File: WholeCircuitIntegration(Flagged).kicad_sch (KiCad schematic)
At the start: 18 parts, among them J1 Conn_02x20_Odd_Even, J2 Conn_01x03_Socket, J3 Conn_01x03_Socket, J4 Conn_01x03_Socket, J5 Conn_01x03_Socket, J6 TBP03R2-350-03BE, J7 TBP03R2-350-03BE, J8 TBP03R2-350-03BE, J9 TBP03R2-350-03BE, U1 ADS1115IDGS, U2 BNO055, U3 74LV14

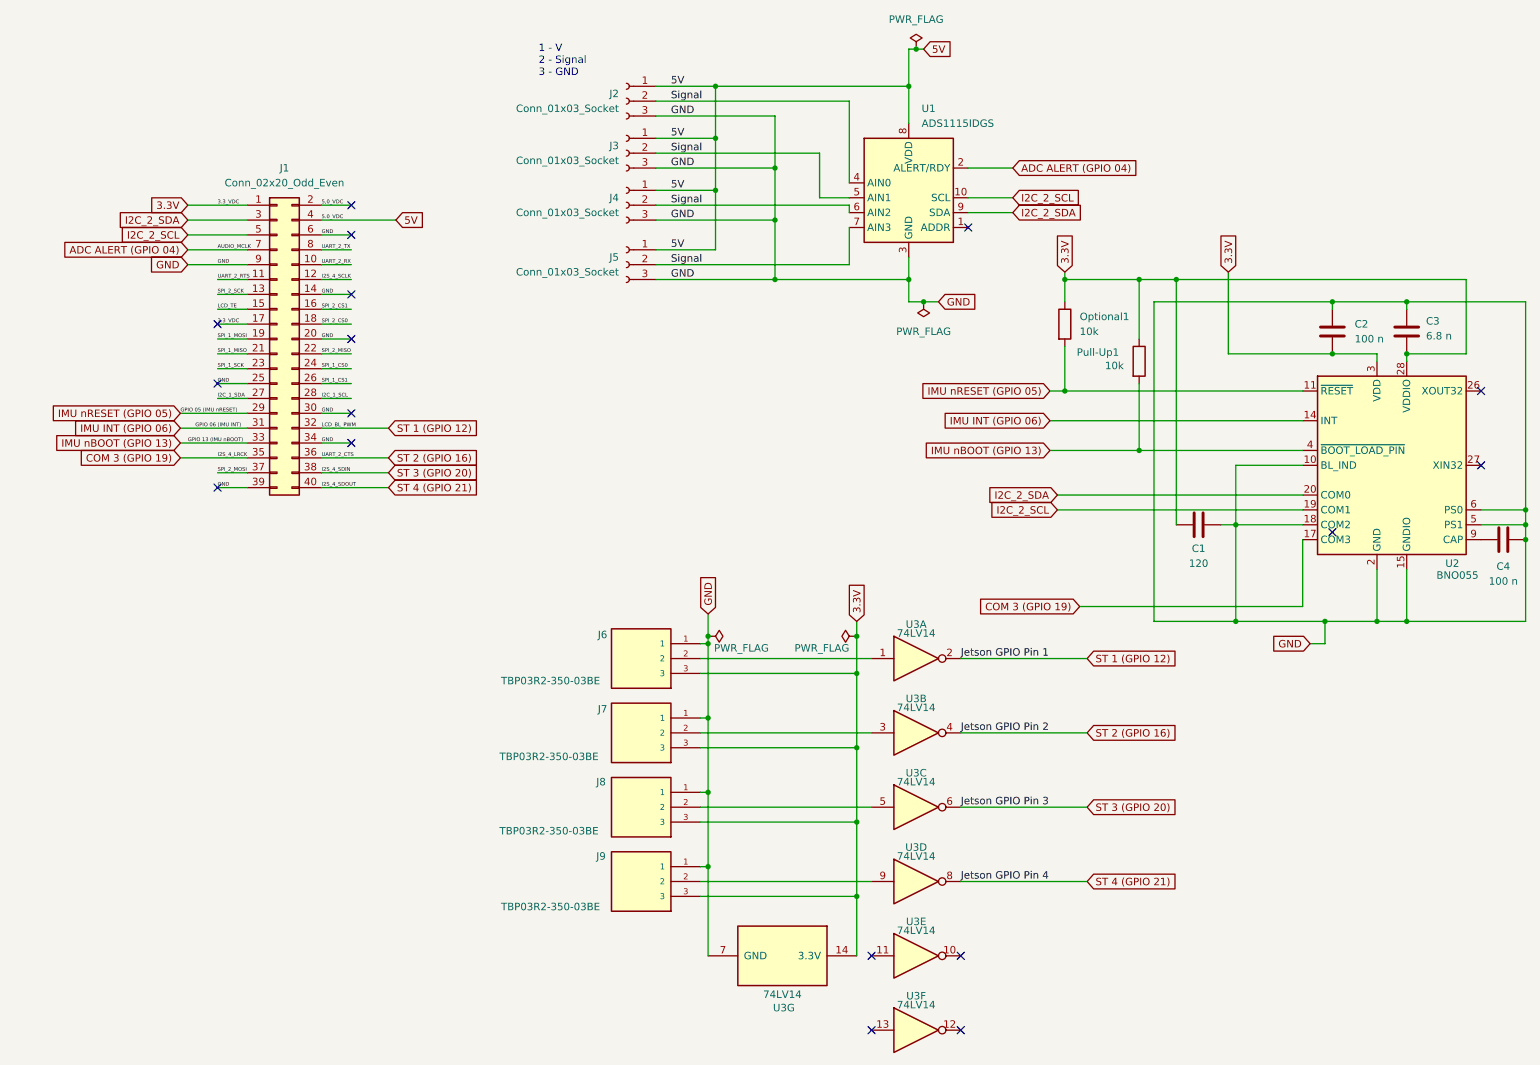
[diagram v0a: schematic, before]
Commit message: Whole Circuit Integration
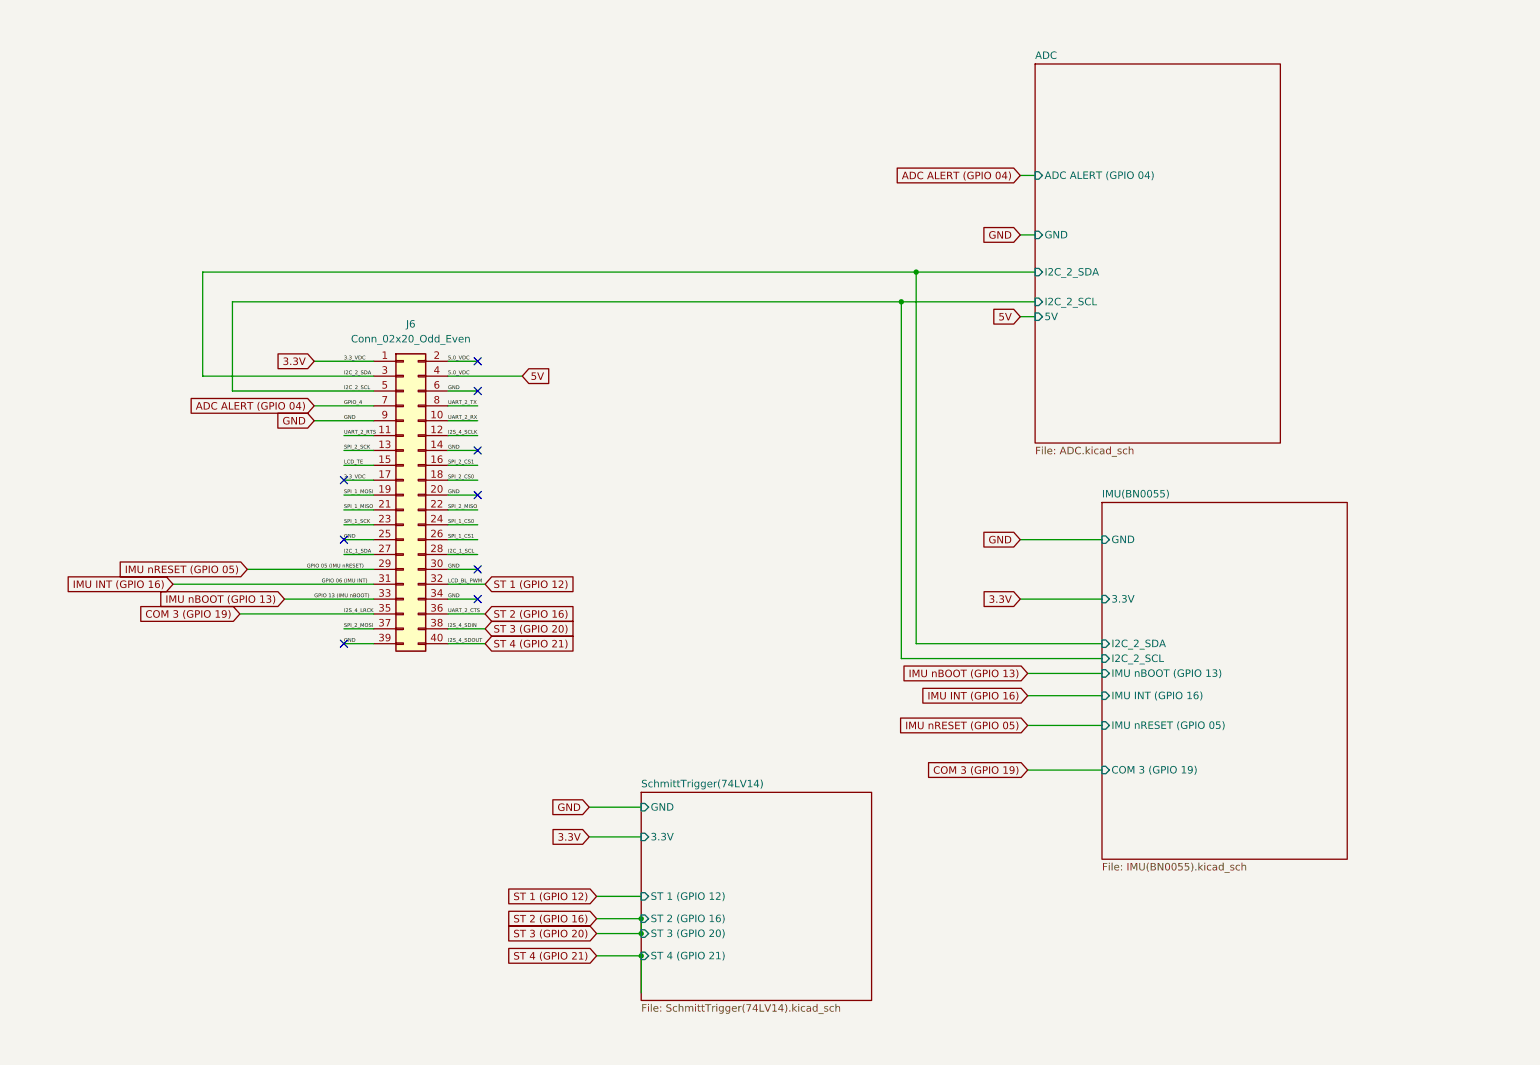
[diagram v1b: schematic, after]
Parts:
- removed C1: 120, Capacitor_SMD:CP_Elec_4x3, symbol Device:C
- removed C2, C4: 100 n, Capacitor_SMD:CP_Elec_4x3, symbol Device:C
- removed C3: 6.8 n, Capacitor_SMD:CP_Elec_4x3, symbol Device:C
- removed J1: Conn_02x20_Odd_Even, symbol Connector_Generic:Conn_02x20_Odd_Even
- removed J2, J3, J4, J5: Conn_01x03_Socket, symbol Connector:Conn_01x03_Socket
- removed J6, J7, J8, J9: TBP03R2-350-03BE, TBP03R2_350_03BE:CUI_TBP03R2-350-03BE, symbol TBP03R2-350-03BE:TBP03R2-350-03BE
- removed Optional1, Pull-Up1: 10k, Resistor_SMD:R_0603_1608Metric_Pad0.98x0.95mm_HandSolder, symbol Device:R
- removed U1: ADS1115IDGS, Package_SO:TSSOP-10_3x3mm_P0.5mm, symbol Analog_ADC:ADS1115IDGS
- removed U2: BNO055, Package_LGA:LGA-28_5.2x3.8mm_P0.5mm, symbol Sensor_Motion:BNO055
- removed U3: 74LV14, Package_DIP:DIP-12_W7.62mm, symbol 74xx:74LV14
- added J6: Conn_02x20_Odd_Even, symbol Connector_Generic:Conn_02x20_Odd_Even
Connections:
- net 3.3V: now also J6.1 (Pin_1), J6.17 (Pin_17)
- net 5,0_VDC: now also J6.2 (Pin_2)
- net 5V: now also J6.4 (Pin_4)
- net ADC ALERT (GPIO 04): now also J6.7 (Pin_7)
- net COM 3 (GPIO 19): now also J6.35 (Pin_35)
- net GND: now also J6.14 (Pin_14), J6.20 (Pin_20), J6.25 (Pin_25), J6.30 (Pin_30), J6.34 (Pin_34), J6.39 (Pin_39), J6.6 (Pin_6), J6.9 (Pin_9)
- net I2C_1_SCL: now also J6.28 (Pin_28)
- net I2C_1_SDA: now also J6.27 (Pin_27)
- net I2C_2_SCL: now also J6.5 (Pin_5)
- net I2C_2_SDA: now also J6.3 (Pin_3)
- net I2S_4_SCLK: now also J6.12 (Pin_12)
- net IMU nBOOT (GPIO 13): now also J6.33 (Pin_33)
- net IMU nRESET (GPIO 05): now also J6.29 (Pin_29)
- net LCD_TE: now also J6.15 (Pin_15)
- net SPI_1_CS0: now also J6.24 (Pin_24)
- net SPI_1_CS1: now also J6.26 (Pin_26)
- net SPI_1_MISO: now also J6.21 (Pin_21)
- net SPI_1_MOSI: now also J6.19 (Pin_19)
- net SPI_1_SCK: now also J6.23 (Pin_23)
- net SPI_2_CS0: now also J6.18 (Pin_18)
- net SPI_2_CS1: now also J6.16 (Pin_16)
- net SPI_2_MISO: now also J6.22 (Pin_22)
- net SPI_2_MOSI: now also J6.37 (Pin_37)
- net SPI_2_SCK: now also J6.13 (Pin_13)
- net ST 1 (GPIO 12): now also J6.32 (Pin_32)
- net ST 2 (GPIO 16): now also J6.36 (Pin_36), J6.38 (Pin_38)
- net ST 4 (GPIO 21): now also J6.40 (Pin_40)
- net UART_2_RTS: now also J6.11 (Pin_11)
- net UART_2_RX: now also J6.10 (Pin_10)
- net UART_2_TX: now also J6.8 (Pin_8)
- new net IMU INT (GPIO 16): J6.31 (Pin_31)
- no-connect marks 17 -> 9
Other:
- added sheet ADC (ADC.kicad_sch)
- added sheet IMU(BN0055) (IMU(BN0055).kicad_sch)
- added sheet SchmittTrigger(74LV14) (SchmittTrigger(74LV14).kicad_sch)
- note removed: "1 - V 2 - Signal 3 - GND"
